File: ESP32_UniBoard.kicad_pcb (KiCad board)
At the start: 4 copper layers, 34 x 52.3 mm, 30 parts, among them J1 USB_C_Receptacle_USB2.0, J2 Conn_01x06_Socket, J3 Hirose DF40C, SW1 SW_Push, SW2 SW_Push, U1 ESP32-S3-WROOM-1, U2 AZ1117-3.3, U3 USBLC6-2SC6

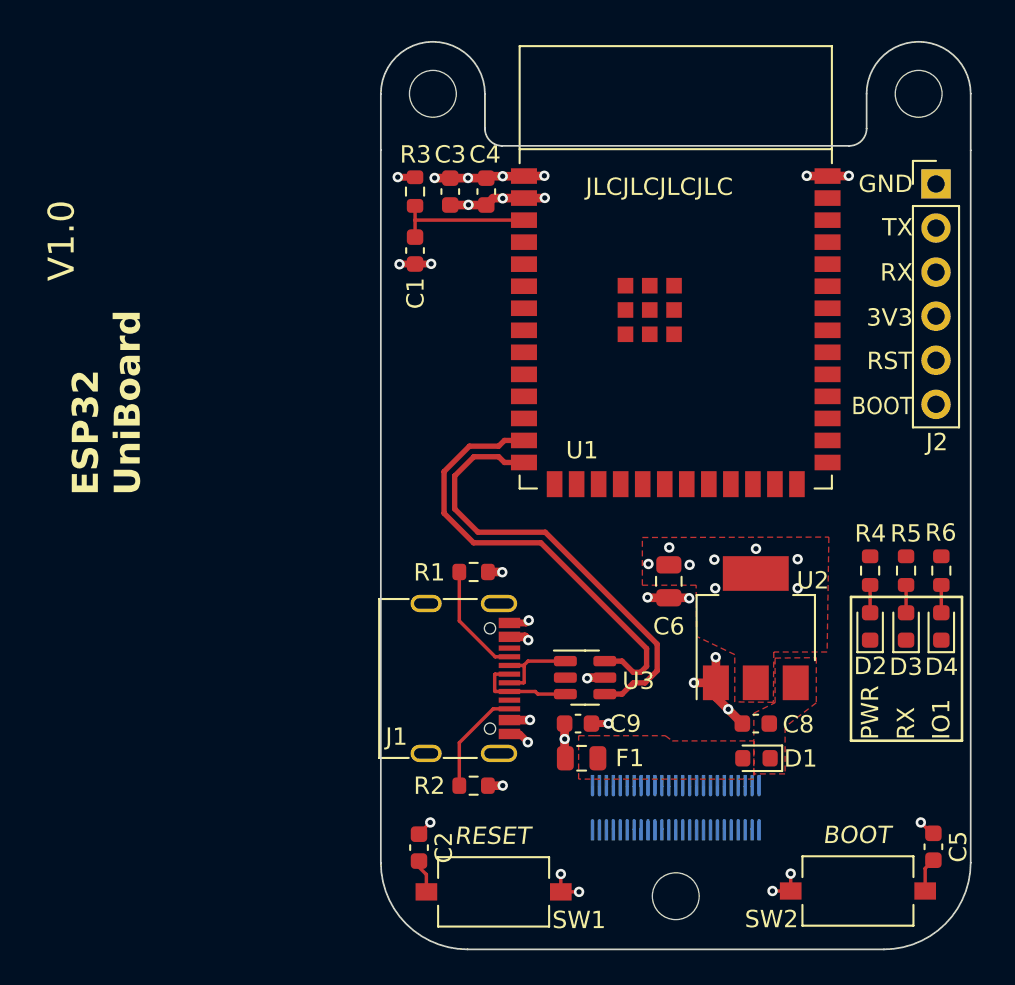
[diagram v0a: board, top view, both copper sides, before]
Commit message: Additional routing~
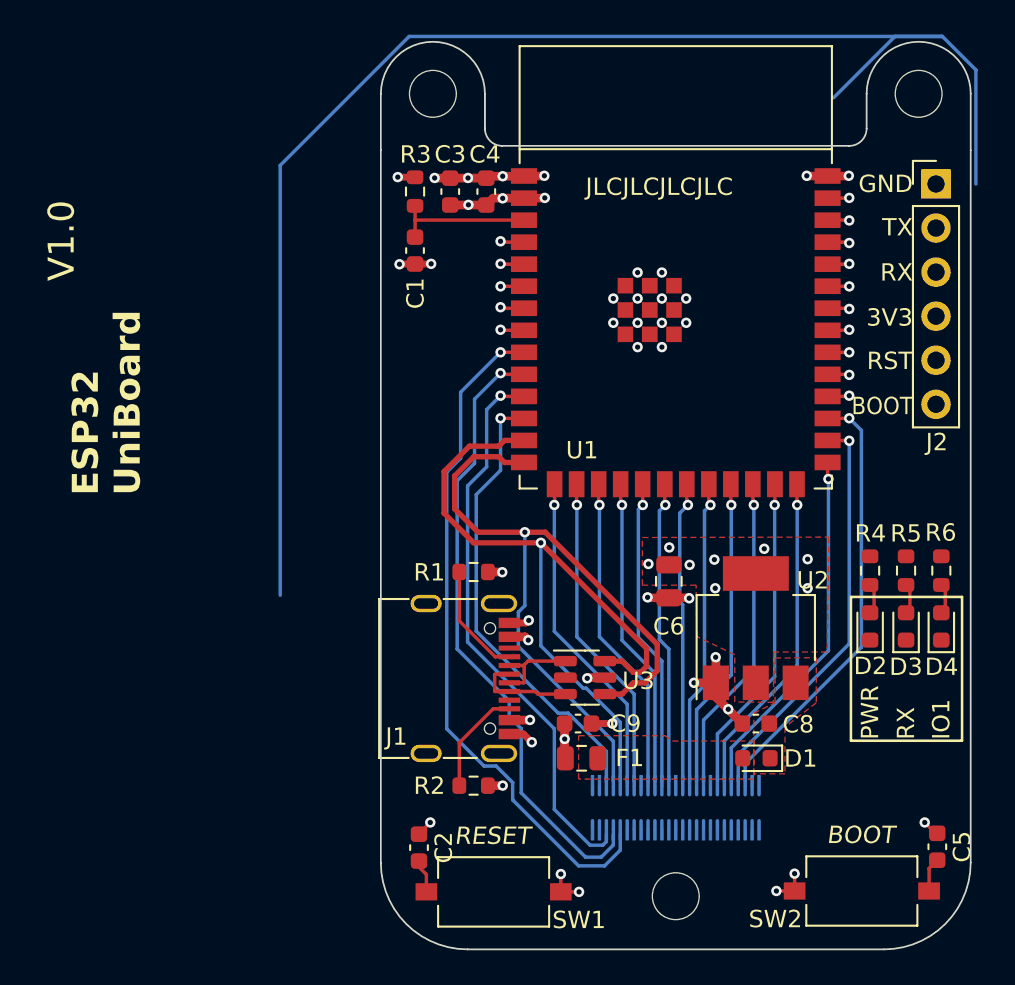
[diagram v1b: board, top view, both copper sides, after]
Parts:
- moved C5 0.22 mm to (136.2, 90.7)
- moved SW2 0.22 mm to (131.8, 93.3)
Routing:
- net (no net): track 0.00 -> 83.1 mm
- net /GPIO16: track 0.00 -> 39.5 mm, vias 0 -> 1
- net /GPIO17: track 0.00 -> 35.9 mm, vias 0 -> 1
- net /GPIO18: track 0.00 -> 32.4 mm, vias 0 -> 1
- net /GPIO8: track 0.00 -> 26.3 mm, vias 0 -> 1
- net /GPIO36: track 0.00 -> 25.2 mm, vias 0 -> 1
- net /GPIO35: track 0.00 -> 23.5 mm, vias 0 -> 1
- net /BOOT: track 1.97 -> 22.7 mm, vias 0 -> 1
- net /GPIO3: track 0.00 -> 18.9 mm, vias 0 -> 1
- net /GPIO45: track 0.00 -> 18.9 mm, vias 0 -> 1
- net /GPIO48: track 0.00 -> 18.5 mm, vias 0 -> 1
- net /GPIO46: track 0.00 -> 18.5 mm, vias 0 -> 1
- net /GPIO47: track 0.00 -> 18.3 mm, vias 0 -> 1
- net /GPIO9: track 0.00 -> 18.3 mm, vias 0 -> 1
- net /GPIO21: track 0.00 -> 17.9 mm, vias 0 -> 1
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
